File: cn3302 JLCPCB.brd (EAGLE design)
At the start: 54 x 20 mm, 20 parts, among them M1 CN3302SOP-8, T1 AOD9N50

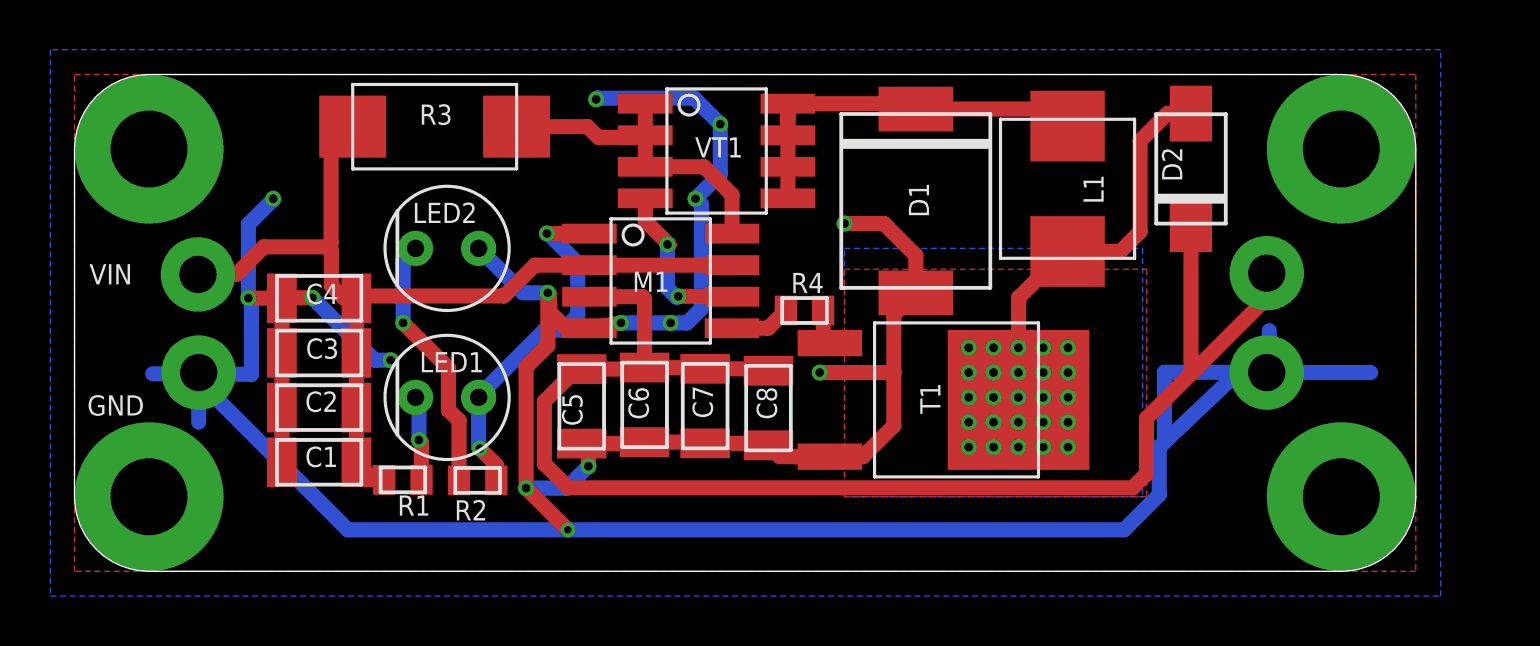
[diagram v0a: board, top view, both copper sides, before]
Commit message: футпринт lid
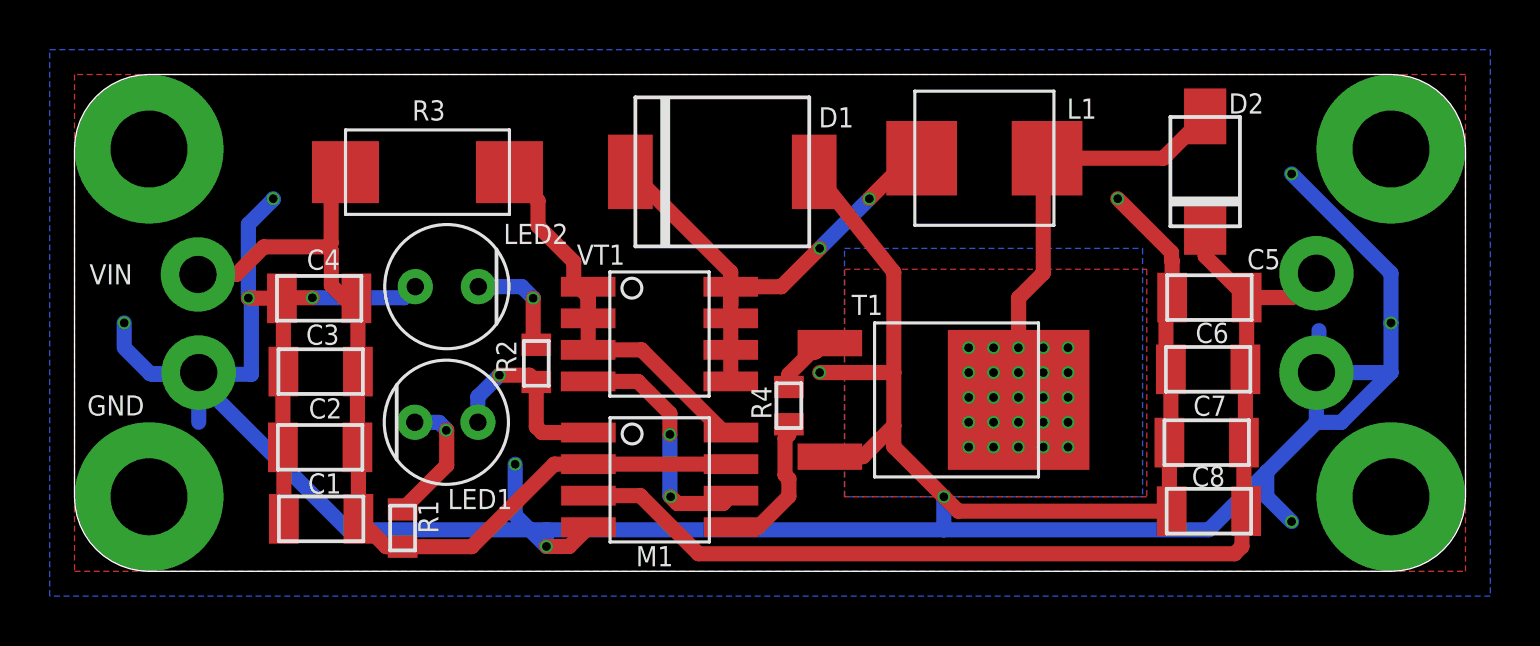
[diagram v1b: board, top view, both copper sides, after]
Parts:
- moved C5 25.6 mm to (46.7, 12.0), turned to 0 degrees
- moved C6 22.7 mm to (46.6, 9.13), turned to 0 degrees
- moved C7 20.2 mm to (46.6, 6.18), turned to 0 degrees
- moved C8 18.2 mm to (46.7, 3.42), turned to 0 degrees
- moved M1 8.01 mm to (24.6, 4.68)
- moved D1 7.88 mm to (27.1, 17.1), turned to 0 degrees
- moved VT1 7.72 mm to (24.6, 10.6)
- moved R2 5.27 mm to (19.6, 9.37), turned to 90 degrees
- moved R4 3.88 mm to (29.8, 7.67), turned to 90 degrees
- moved L1 3.57 mm to (37.6, 17.6), turned to 0 degrees
- moved C1 2.28 mm to (10.9, 3.11)
- moved R1 1.94 mm to (14.2, 2.74), turned to 90 degrees
- moved R3 1.85 mm to (15.2, 17.1)
- moved C2 1.60 mm to (10.9, 5.99)
- moved LED2 1.54 mm to (16.0, 12.5), turned to 0 degrees
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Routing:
- net 8.4V: track 59.3 -> 45.3 mm
- net N$5: track 14.6 -> 7.85 mm, vias 2 -> 1
- net N$2: track 10.5 -> 4.33 mm
- net N$9: track 16.4 -> 20.9 mm, vias 0 -> 2
- net N$6: track 13.5 -> 16.9 mm
- net N$4: track 2.47 -> 5.87 mm
- net N$3: track 6.86 -> 9.89 mm
- net N$1: track 3.42 -> 5.36 mm
- net N$8: track 1.43 -> 2.92 mm
- net S$1: track 0.00 -> 0.90 mm, vias 0 -> 1
- net N$10: track 16.7 -> 17.3 mm
- net GND: track 157.8 -> 157.4 mm, vias 15 -> 11
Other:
- board size 54 x 20 mm -> 56 x 20 mm
